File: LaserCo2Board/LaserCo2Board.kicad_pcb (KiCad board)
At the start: 2 copper layers, 106.8 x 58.5 mm, 137 parts, among them J1 Y VREF, J10 LASER, J11 X MOTOR, J12 Y1 MOTOR, J13 WATER FLOW, J14 Y2 MOTOR, J15 LASER P, J16 X LIMIT1, J17 X LIMIT2, J18 Y LIMIT1, J19 Y LIMIT2, J2 X VREF, J20 D SWITCH, J3 JTAG, J4 USB, J5 POWER IN, J6 FAN1, J7 FAN2, J8 FAN3, J9 PUMP, Q1 BSS138, Q2 BSS138, SW1 SW_PUSH, SW2 SWITCH_INV, U1 STM32F20XR, U2 A4982SLPTR, U3 A4982SLPTR, U4 LD1117S33TR, U5 74HC08A, U6 MCP4725, U7 MCP44X1, U8 74HC1G00, X1 CRYSTAL_4PIN, X2 CRYSTAL

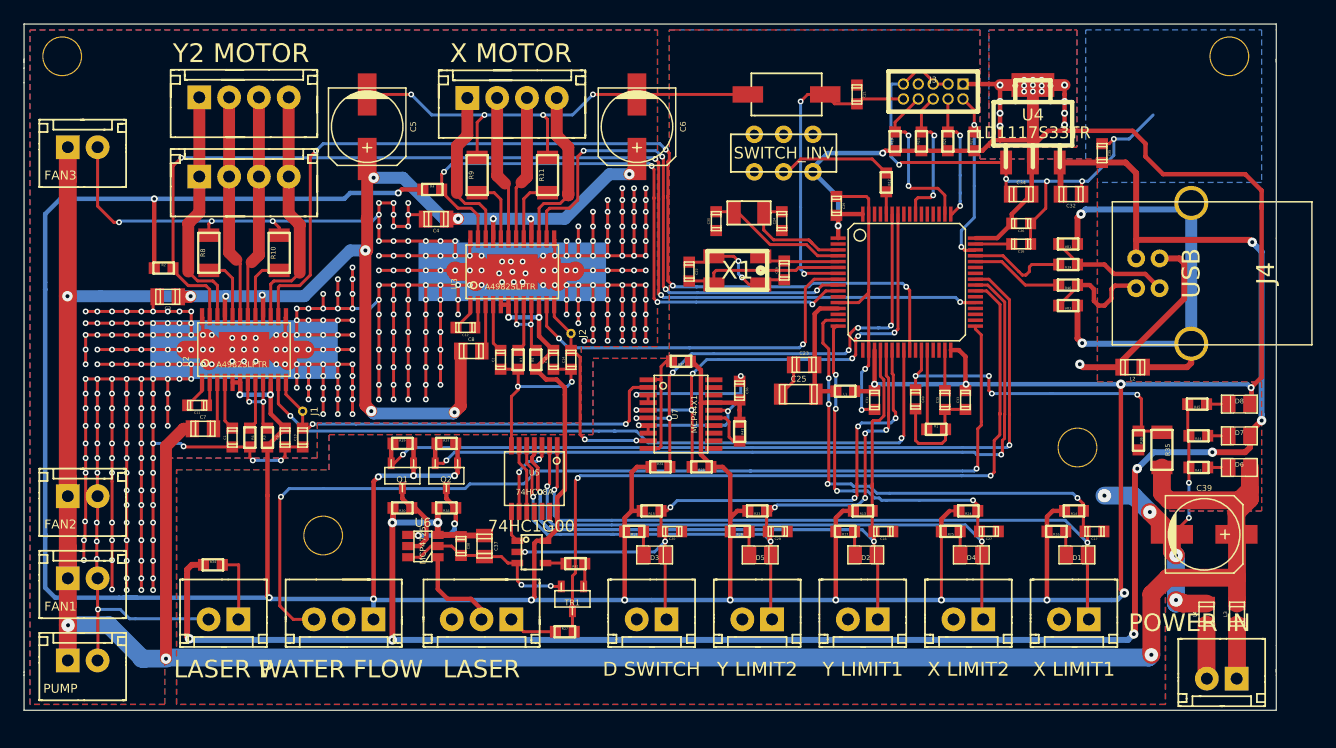
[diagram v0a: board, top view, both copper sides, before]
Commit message: ノイズ対策2
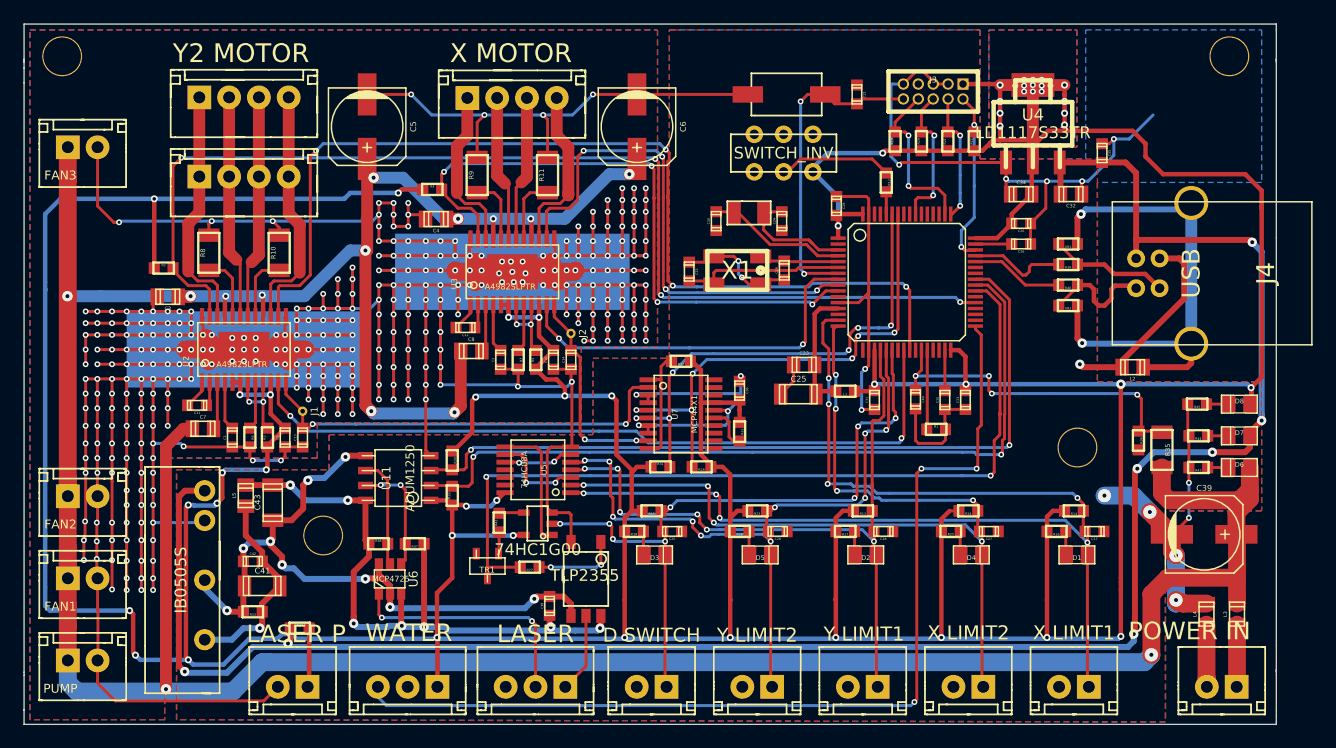
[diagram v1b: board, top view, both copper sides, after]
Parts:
- removed C37: 10u, C_0805
- removed Q1, Q2: BSS138, SOT-23
- added C41: 10u, C_1206, F.Cu at (49.8, 75.4)
- added C42: 0u1, C_0603, F.Cu at (49.0, 73.3)
- added C43: 10u, C_1206, F.Cu at (50.7, 68.3)
- added L5: inductor, C_0805, F.Cu at (48.4, 67.7)
- added R33: 1k, R_0603, F.Cu at (49.0, 77.6)
- added U10: IB0505S, IB0505S, F.Cu at (44.9, 74.9)
- added U11: ADUM1250, SOIC-8, F.Cu at (61.4, 66.2)
- added U9: TLP2355, TLP2355, F.Cu at (77.4, 74.8)
- J13: value WATER FLOW -> WATER
- R27: value 22R -> 220R
- R29, R30, R37, R38: value 10k -> 4k7
- moved R34 9.16 mm to (53.0, 79.0)
- moved C38 9.11 mm to (74.3, 77.1), turned to 90 degrees
- moved R37 8.97 mm to (62.8, 71.8), turned to 180 degrees
- moved J15 8.24 mm to (52.4, 84.0)
- moved J13 7.92 mm to (62.2, 84.0)
- moved TR1 7.77 mm to (69.0, 73.7)
- moved R41 7.38 mm to (70.0, 70.0), turned to 90 degrees
- moved J10 7.36 mm to (73.1, 84.0)
- moved R38 6.55 mm to (59.7, 71.8), turned to 0 degrees
- moved R27 6.26 mm to (72.6, 73.8), turned to 180 degrees
- moved R29 6.15 mm to (66.0, 67.7), turned to 90 degrees
- moved R30 5.87 mm to (66.0, 64.7), turned to 270 degrees
- moved J16 5.75 mm to (119.0, 84.0)
- moved J17 5.75 mm to (110.0, 84.0)
- moved J18 5.75 mm to (101.0, 84.0)
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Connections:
- C38 pad 1: GND -> DGND
- C38 pad 2: VBUS -> D5V
- R27 pad 1: LASER_OUT_CONN -> N-0000045
- R29 pad 1: SCL1 -> +3.3V
- R29 pad 2: +3.3V -> SDA1
- R30 pad 1: N-0000057 -> +3.3V
- R30 pad 2: VBUS -> SCL1
- R37 pad 1: SDA1 -> D5V
- R37 pad 2: +3.3V -> N-0000059
- R38 pad 1: N-0000059 -> D5V
- R38 pad 2: VBUS -> N-0000058
- U6 pad 2: GND -> DGND
- U6 pad 3: VBUS -> D5V
- U6 pad 5: N-0000057 -> N-0000058
- U6 pad 6: GND -> DGND
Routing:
- net DGND: track 0.00 -> 58.8 mm, vias 0 -> 9
- net D5V: track 0.00 -> 55.6 mm, vias 0 -> 7
- net +3.3V: track 509.1 -> 555.6 mm, vias 43 -> 52
- net Y_LIMIT1: track 94.8 -> 61.5 mm, vias 2 -> 6
- net GND: track 842.4 -> 863.0 mm, vias 390 -> 387
- net N-00000125: track 0.00 -> 17.4 mm, vias 0 -> 1
- net LASER_ANALOG: track 8.01 -> 20.8 mm, vias 0 -> 2
- net N-0000058: track 0.00 -> 9.45 mm
- net N-0000090: track 2.71 -> 11.1 mm
- net VBUS: track 190.0 -> 181.8 mm, vias 9 -> 7
- net N-0000045: track 0.00 -> 7.35 mm, vias 0 -> 2
- net N-0000057: track 7.19 -> 0.00 mm
- net LASER_OUT: track 66.4 -> 72.4 mm
- net X_LIMIT1: track 105.9 -> 99.9 mm, vias 6 -> 8
- net V_IN: track 299.0 -> 303.8 mm, vias 15 -> 14
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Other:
- board size 106.8 x 58.5 mm -> 106.8 x 59.7 mm

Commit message: 元に戻す
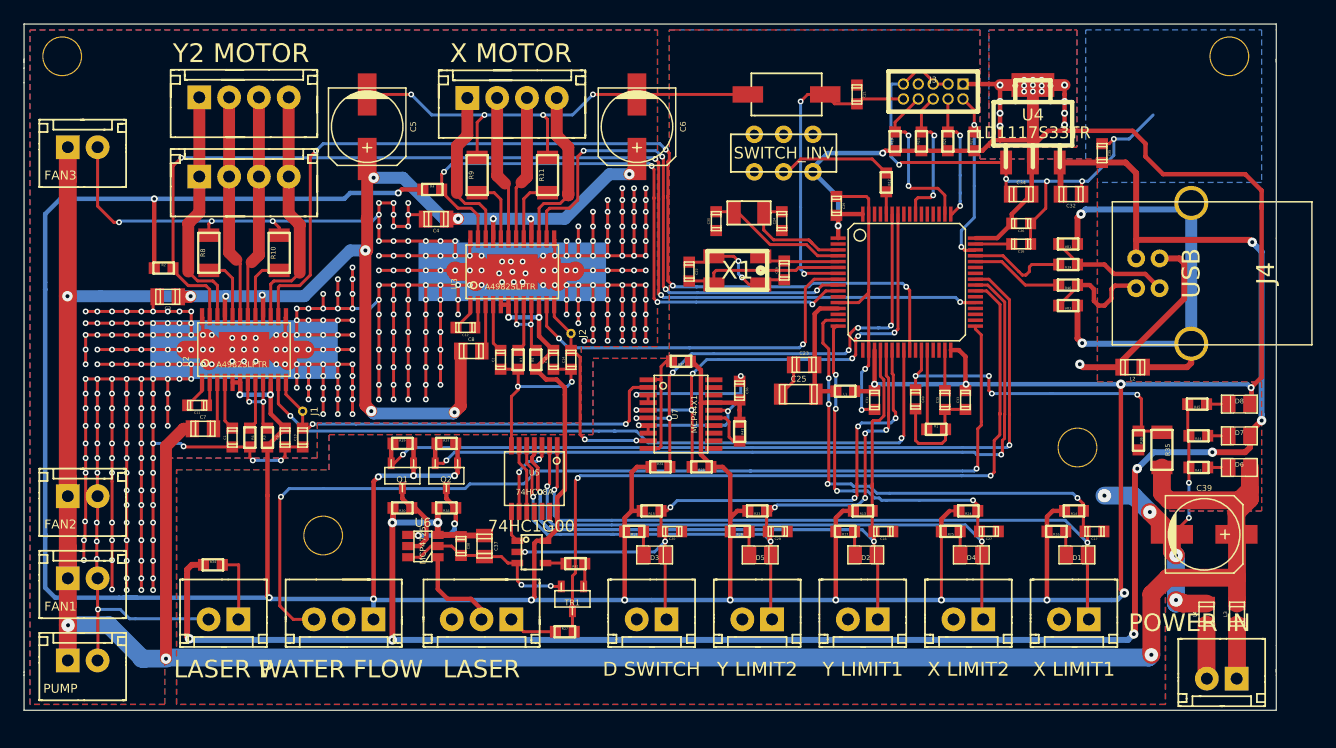
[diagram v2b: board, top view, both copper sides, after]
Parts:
- removed C41, C43: 10u, C_1206
- removed C42: 0u1, C_0603
- removed L5: inductor, C_0805
- removed R33: 1k, R_0603
- removed U10: IB0505S, IB0505S
- removed U11: ADUM1250, SOIC-8
- removed U9: TLP2355, TLP2355
- added C37: 10u, C_0805, F.Cu at (68.8, 72.0)
- added Q1: BSS138, SOT-23, F.Cu at (61.8, 66.0)
- added Q2: BSS138, SOT-23, F.Cu at (65.5, 66.0)
- J13: value WATER -> WATER FLOW
- R27: value 220R -> 22R
- R29, R30, R37, R38: value 4k7 -> 10k
- moved R34 9.16 mm to (45.6, 73.6)
- moved C38 9.11 mm to (66.8, 72.0), turned to 270 degrees
- moved R37 8.97 mm to (65.5, 63.2), turned to 0 degrees
- moved J15 8.24 mm to (46.5, 78.2)
- moved J13 7.92 mm to (56.8, 78.2)
- moved TR1 7.77 mm to (76.2, 76.5)
- moved R41 7.38 mm to (76.5, 73.5), turned to 180 degrees
- moved J10 7.36 mm to (68.5, 78.2)
- moved R38 6.55 mm to (65.5, 68.8), turned to 180 degrees
- moved R27 6.26 mm to (75.6, 79.3), turned to 0 degrees
- moved R29 6.15 mm to (61.8, 63.2), turned to 0 degrees
- moved R30 5.87 mm to (61.8, 68.8), turned to 180 degrees
- moved J16 5.75 mm to (119.0, 78.2)
- moved J17 5.75 mm to (110.0, 78.2)
- moved J18 5.75 mm to (101.0, 78.2)
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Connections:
- C38 pad 1: DGND -> GND
- C38 pad 2: D5V -> VBUS
- R27 pad 1: N-0000045 -> LASER_OUT_CONN
- R29 pad 1: +3.3V -> SCL1
- R29 pad 2: SDA1 -> +3.3V
- R30 pad 1: +3.3V -> N-0000057
- R30 pad 2: SCL1 -> VBUS
- R37 pad 1: D5V -> SDA1
- R37 pad 2: N-0000059 -> +3.3V
- R38 pad 1: D5V -> N-0000059
- R38 pad 2: N-0000058 -> VBUS
- U6 pad 2: DGND -> GND
- U6 pad 3: D5V -> VBUS
- U6 pad 5: N-0000058 -> N-0000057
- U6 pad 6: DGND -> GND
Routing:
- net DGND: track 58.8 -> 0.00 mm, vias 9 -> 0
- net D5V: track 55.6 -> 0.00 mm, vias 7 -> 0
- net +3.3V: track 555.6 -> 509.1 mm, vias 52 -> 43
- net Y_LIMIT1: track 61.5 -> 94.8 mm, vias 6 -> 2
- net GND: track 863.0 -> 842.4 mm, vias 387 -> 390
- net N-00000125: track 17.4 -> 0.00 mm, vias 1 -> 0
- net LASER_ANALOG: track 20.8 -> 8.01 mm, vias 2 -> 0
- net N-0000058: track 9.45 -> 0.00 mm
- net N-0000081: track 11.1 -> 2.71 mm
- net VBUS: track 181.8 -> 190.0 mm, vias 7 -> 9
- net N-0000045: track 7.35 -> 0.00 mm, vias 2 -> 0
- net N-0000057: track 0.00 -> 7.19 mm
- net LASER_OUT: track 72.4 -> 66.4 mm
- net X_LIMIT1: track 99.9 -> 105.9 mm, vias 8 -> 6
- net V_IN: track 303.8 -> 299.0 mm, vias 14 -> 15
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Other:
- board size 106.8 x 59.7 mm -> 106.8 x 58.5 mm
